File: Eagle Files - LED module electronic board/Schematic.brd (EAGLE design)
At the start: 30.5 x 30.5 mm, 14 parts, among them IC1 AMS1117-1.5, IC2 LM358N, J1 2.54 CONN, J2 2.54 CONN, Q1 P16NF06L

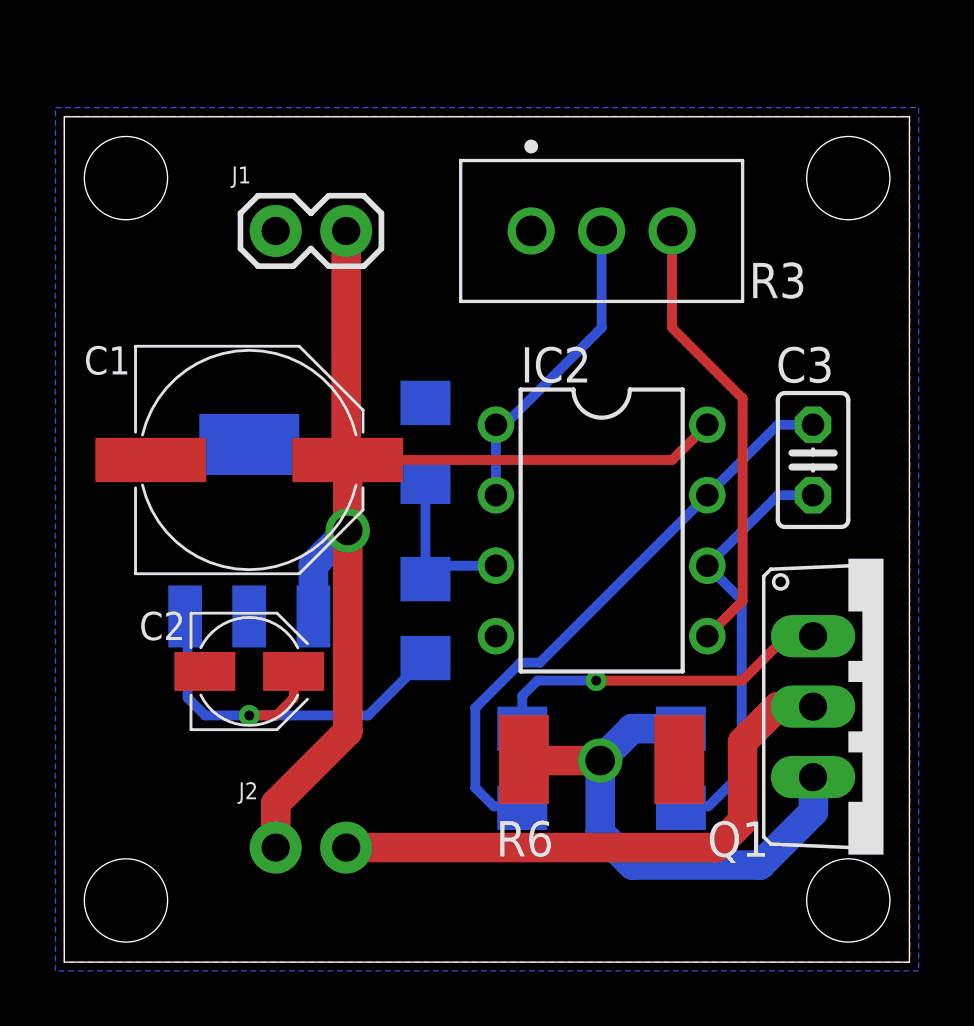
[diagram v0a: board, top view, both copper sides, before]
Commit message: Update
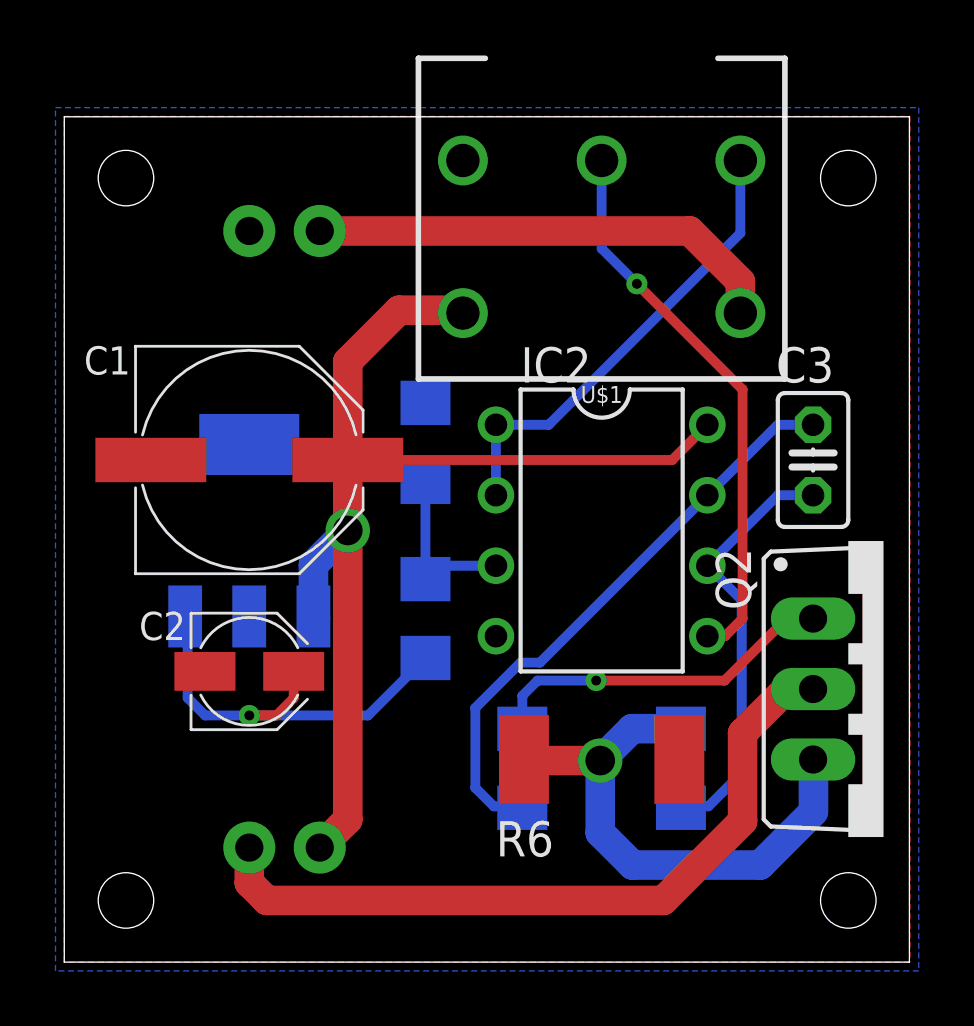
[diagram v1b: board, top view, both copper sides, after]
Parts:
- removed J1, J2: 2.54 CONN, SparkFun-Connectors:1X02
- removed Q1: P16NF06L, adafruit:TO220V
- removed R3: 10k, LED-microscope-library:HDRV3W64P254_1X3_1016X508X838B
- added Q2: P16NF06L, transistor-power:TO220BV
- added U$1: (no value), untitled:POT-SWITCH-PTH
- added U$3, U$4: (no value), untitled:1X02_NO_SILK
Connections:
- new net N$10: IC2.5, U$1.2
- net GND: now also U$1.3, U$3.2; no longer J1.1, R3.1
- net N$1: now also U$1.5, U$3.1; no longer IC2.5, R3.3
- net N$4: now also U$1.1; no longer R3.2
- net N$5: now also Q2.D, U$4.1; no longer J2.2, Q1.2
- net N$7: now also Q2.G; no longer Q1.1
- net N$9: now also Q2.S; no longer Q1.3
- net VCC: now also U$1.4, U$4.2; no longer J1.2, J2.1
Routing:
- net N$10: track 0.00 -> 20.1 mm, vias 0 -> 1
- net N$5: track 20.6 -> 26.9 mm
- net N$4: track 11.3 -> 17.1 mm
- net N$1: track 16.2 -> 17.1 mm
- net N$9: track 19.0 -> 19.6 mm
